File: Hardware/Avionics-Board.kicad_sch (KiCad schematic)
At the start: 9 parts, among them J1 USB-C, U1 ICM-20948, U2 BMP390

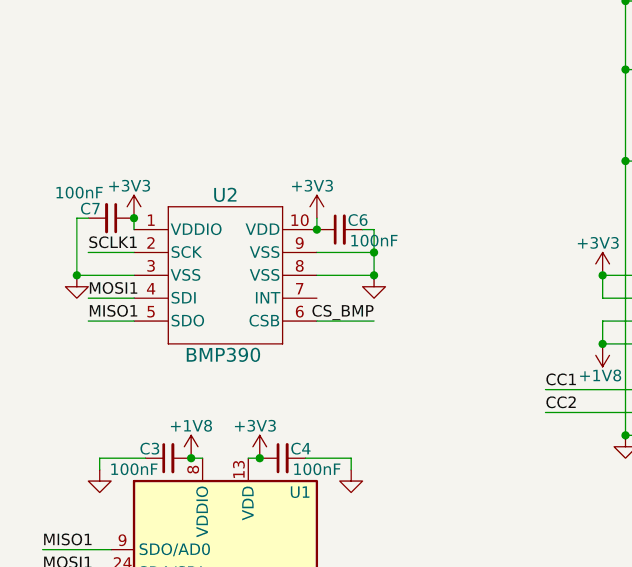
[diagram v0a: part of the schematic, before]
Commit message: Day-5
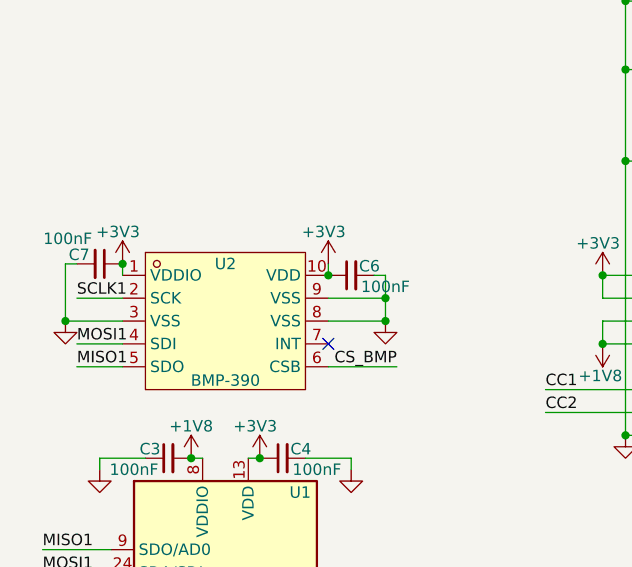
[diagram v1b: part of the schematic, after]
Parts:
- removed U2: BMP390, Avionics-Board:BMP390, symbol BMP390:BMP390
- added U2: BMP-390, easyeda2kicad:LGA-10_L2.0-W2.0-P0.50-BL, symbol easyeda2kicad:BMP390_C5124834
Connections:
- net +3V3: now also U2.1 (VDDIO), U2.10 (VDD)
- net CS_BMP: now also U2.6 (CSB)
- net GND: now also U2.3 (VSS), U2.8 (VSS), U2.9 (VSS)
- net MISO1: now also U2.5 (SDO)
- net MOSI1: now also U2.4 (SDI)
- net SCLK1: now also U2.2 (SCK)
- no-connect marks 2 -> 3
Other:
- moved on the sheet: C6, C7
